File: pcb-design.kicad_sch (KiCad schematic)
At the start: 28 parts, among them J1 USB_C_Receptacle_USB2.0_16P, J2 Conn_01x04_Pin, SW1 SW_Push, SW2 SW_Push, U1 RP2040, U2 W25Q16JVSS, U3 USBLC6-2SC6, U4 SPX3819M5-L-3-3, Y1 12Mhz

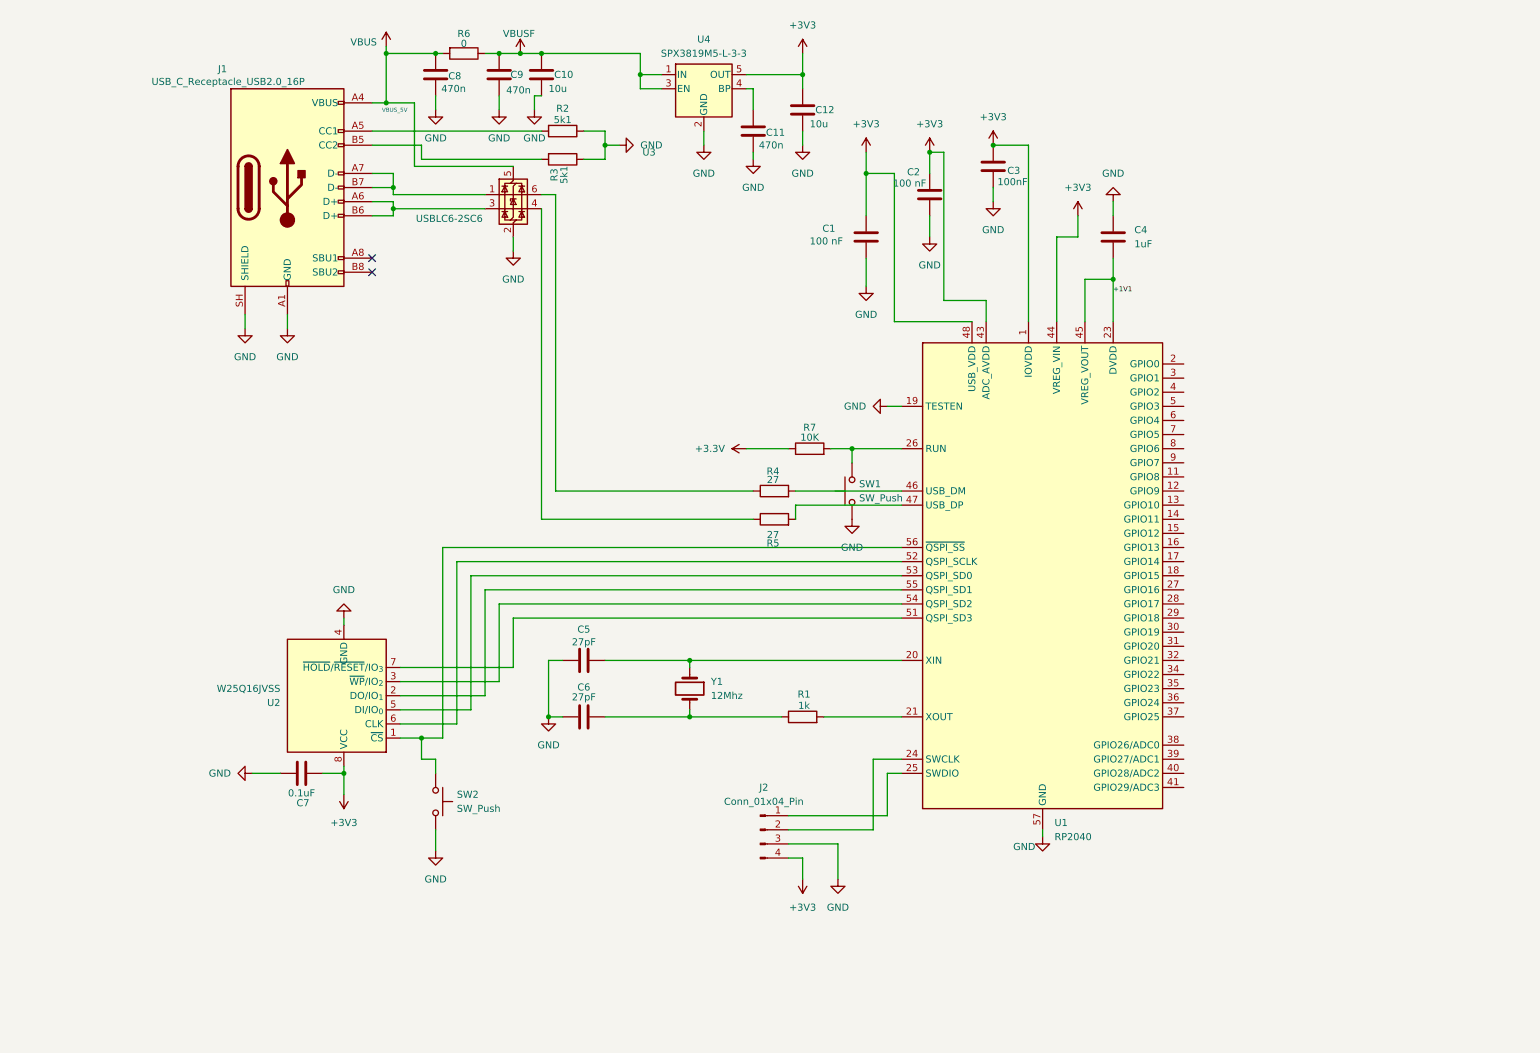
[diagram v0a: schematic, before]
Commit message: File updated
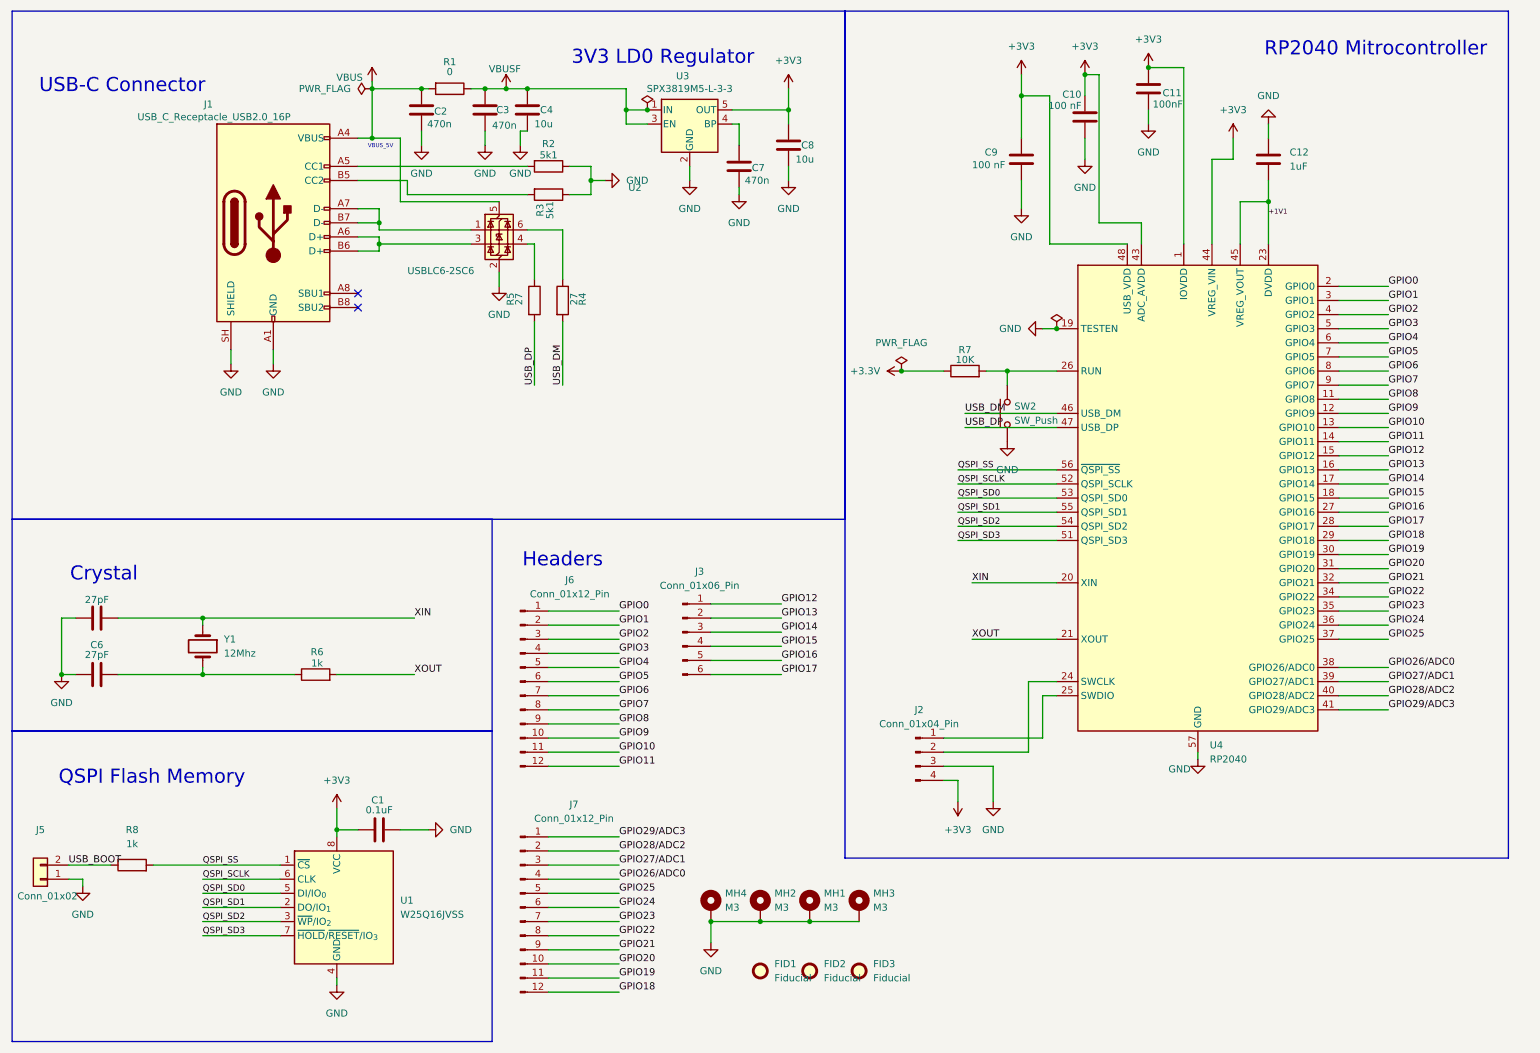
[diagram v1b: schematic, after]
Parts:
- removed SW2: SW_Push, symbol Switch:SW_Push
- added FID1, FID2, FID3: Fiducial, Fiducial:Fiducial_1mm_Mask2mm, symbol Mechanical:Fiducial
- added J3: Conn_01x06_Pin, Connector_PinSocket_2.54mm:PinSocket_1x06_P2.54mm_Vertical, symbol Connector:Conn_01x06_Pin
- added J5: Conn_01x02, Connector_PinSocket_2.54mm:PinSocket_1x02_P2.54mm_Vertical, symbol Connector_Generic:Conn_01x02
- added J6, J7: Conn_01x12_Pin, Connector_PinSocket_2.54mm:PinSocket_1x12_P2.54mm_Vertical, symbol Connector:Conn_01x12_Pin
- added MH1, MH2, MH3, MH4: M3, MountingHole:MountingHole_3.2mm_M3_Pad_Via, symbol Mechanical:MountingHole_Pad
- added R8: 1k, Resistor_SMD:R_0805_2012Metric, symbol Device:R
- C1: renamed from C7; footprint (none) -> Capacitor_SMD:C_0603_1608Metric
- C10: renamed from C2; footprint (none) -> Capacitor_SMD:C_0603_1608Metric
- C11: renamed from C3; footprint (none) -> Capacitor_SMD:C_0603_1608Metric
- C12: renamed from C4; footprint (none) -> Capacitor_SMD:C_0805_2012Metric
- C2: renamed from C8; footprint (none) -> Capacitor_SMD:C_0805_2012Metric
- C3: renamed from C9; footprint (none) -> Capacitor_SMD:C_0805_2012Metric
- C4: renamed from C10; footprint (none) -> Capacitor_SMD:C_0805_2012Metric
- C5, C6: footprint (none) -> Capacitor_SMD:C_0805_2012Metric
- C7: renamed from C11; footprint (none) -> Capacitor_SMD:C_0805_2012Metric
- C8: renamed from C12; footprint (none) -> Capacitor_SMD:C_0805_2012Metric
- C9: renamed from C1; footprint (none) -> Capacitor_SMD:C_0603_1608Metric
- J1: footprint (none) -> Connector_USB:USB_C_Receptacle_HRO_TYPE-C-31-M-12
- J2: footprint (none) -> Connector_PinSocket_2.54mm:PinSocket_1x04_P2.54mm_Vertical
- R1: renamed from R6; footprint (none) -> Resistor_SMD:R_0805_2012Metric
- R2, R3, R4, R5, R7: footprint (none) -> Resistor_SMD:R_0805_2012Metric
- R6: renamed from R1; footprint (none) -> Resistor_SMD:R_0805_2012Metric
- SW2: renamed from SW1; footprint (none) -> Button_Switch_SMD:SW_SPST_SKQG_WithoutStem
- Y1: footprint (none) -> Crystal:Crystal_SMD_3225-4Pin_3.2x2.5mm
- renumbered U2 to U1, U3 to U2, U4 to U3, U1 to U4
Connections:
- net GND: now also J5.1 (Pin_1), MH1.1, MH2.1, MH3.1, MH4.1
- net QSPI_SS: now reaches U1.1 (~{CS}), U4.56 (~{QSPI_SS})
- net QSPI_SS: now also R8.2
- net QSPI_SD1: now reaches U1.2 (DO/IO_{1}), U4.55 (QSPI_SD1)
- net QSPI_SD2: now reaches U1.3 (~{WP}/IO_{2}), U4.54 (QSPI_SD2)
- net QSPI_SD0: now reaches U1.5 (DI/IO_{0}), U4.53 (QSPI_SD0)
- net QSPI_SCLK: now reaches U1.6 (CLK), U4.52 (QSPI_SCLK)
- net QSPI_SD3: now reaches U1.7 (~{HOLD}/~{RESET}/IO_{3}), U4.51 (QSPI_SD3)
- net USB_DP: now reaches R5.2, U4.47 (USB_DP)
- net XOUT: now reaches R6.2, U4.21 (XOUT)
- net XIN: now reaches C5.1, U4.20 (XIN), Y1.1
- net USB_DM: now reaches R4.2, U4.46 (USB_DM)
- net GPIO8: now reaches U4.11 (GPIO8)
- net GPIO8: now also J6.9 (Pin_9)
- net GPIO9: now reaches U4.12 (GPIO9)
- net GPIO9: now also J6.10 (Pin_10)
- net GPIO10: now reaches U4.13 (GPIO10)
- net GPIO10: now also J6.11 (Pin_11)
- net GPIO11: now reaches U4.14 (GPIO11)
- net GPIO11: now also J6.12 (Pin_12)
- net GPIO12: now reaches U4.15 (GPIO12)
- net GPIO12: now also J3.1 (Pin_1)
- net GPIO13: now reaches U4.16 (GPIO13)
- net GPIO13: now also J3.2 (Pin_2)
- net GPIO14: now reaches U4.17 (GPIO14)
- net GPIO14: now also J3.3 (Pin_3)
- net GPIO15: now reaches U4.18 (GPIO15)
- net GPIO15: now also J3.4 (Pin_4)
- net GPIO0: now reaches U4.2 (GPIO0)
- net GPIO0: now also J6.1 (Pin_1)
- net GPIO16: now reaches U4.27 (GPIO16)
- net GPIO16: now also J3.5 (Pin_5)
- net GPIO17: now reaches U4.28 (GPIO17)
- net GPIO17: now also J3.6 (Pin_6)
- net GPIO18: now reaches U4.29 (GPIO18)
- net GPIO18: now also J7.12 (Pin_12)
- net GPIO1: now reaches U4.3 (GPIO1)
- net GPIO1: now also J6.2 (Pin_2)
- net GPIO19: now reaches U4.30 (GPIO19)
- net GPIO19: now also J7.11 (Pin_11)
- net GPIO20: now reaches U4.31 (GPIO20)
- net GPIO20: now also J7.10 (Pin_10)
- net GPIO21: now reaches U4.32 (GPIO21)
- net GPIO21: now also J7.9 (Pin_9)
- net GPIO22: now reaches U4.34 (GPIO22)
- net GPIO22: now also J7.8 (Pin_8)
- net GPIO23: now reaches U4.35 (GPIO23)
- net GPIO23: now also J7.7 (Pin_7)
- net GPIO24: now reaches U4.36 (GPIO24)
- net GPIO24: now also J7.6 (Pin_6)
- net GPIO25: now reaches U4.37 (GPIO25)
- net GPIO25: now also J7.5 (Pin_5)
- net GPIO26/ADC0: now reaches U4.38 (GPIO26/ADC0)
- net GPIO26/ADC0: now also J7.4 (Pin_4)
- net GPIO27/ADC1: now reaches U4.39 (GPIO27/ADC1)
- net GPIO27/ADC1: now also J7.3 (Pin_3)
- net GPIO2: now reaches U4.4 (GPIO2)
- net GPIO2: now also J6.3 (Pin_3)
- net GPIO28/ADC2: now reaches U4.40 (GPIO28/ADC2)
- net GPIO28/ADC2: now also J7.2 (Pin_2)
- net GPIO29/ADC3: now reaches U4.41 (GPIO29/ADC3)
- net GPIO29/ADC3: now also J7.1 (Pin_1)
- net GPIO3: now reaches U4.5 (GPIO3)
- net GPIO3: now also J6.4 (Pin_4)
- net GPIO4: now reaches U4.6 (GPIO4)
- net GPIO4: now also J6.5 (Pin_5)
- net GPIO5: now reaches U4.7 (GPIO5)
- net GPIO5: now also J6.6 (Pin_6)
- net GPIO6: now reaches U4.8 (GPIO6)
- net GPIO6: now also J6.7 (Pin_7)
- net GPIO7: now reaches U4.9 (GPIO7)
- net GPIO7: now also J6.8 (Pin_8)
- new net USB_BOOT: J5.2 (Pin_2), R8.1
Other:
- note added: "3V3 LD0 Regulator"
- note added: "Crystal"
- note added: "Headers"
- note added: "QSPI Flash Memory"
- note added: "RP2040 Mitrocontroller"
- note added: "USB-C Connector"
- moved on the sheet: C1, C10, C11, C12, C2, C3, C4, C6, C7, C8, C9, J1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
